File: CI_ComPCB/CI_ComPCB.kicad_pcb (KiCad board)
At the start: 2 copper layers, 145 x 101 mm, 30 parts, among them J1 Conn_01x15_Female, J10 Conn_01x02_Male, J1001 Conn_01x06_Female, J1002 Conn_01x06_Female, J1003 Conn_02x04_Odd_Even, J11 Conn_01x02_Male, J12 Conn_01x01_Female, J13 Conn_01x01_Female, J2 Conn_01x02_Male, J4 Conn_01x15_Female, J6 Conn_01x02_Male, J7 Conn_01x03_Male, J8 RJ45_LED_Shielded, J9 RJ45_LED_Shielded, Q1 IRF9540N, Q2 IRF9540N, U1 Boost_Converter, U1001 ESP32s

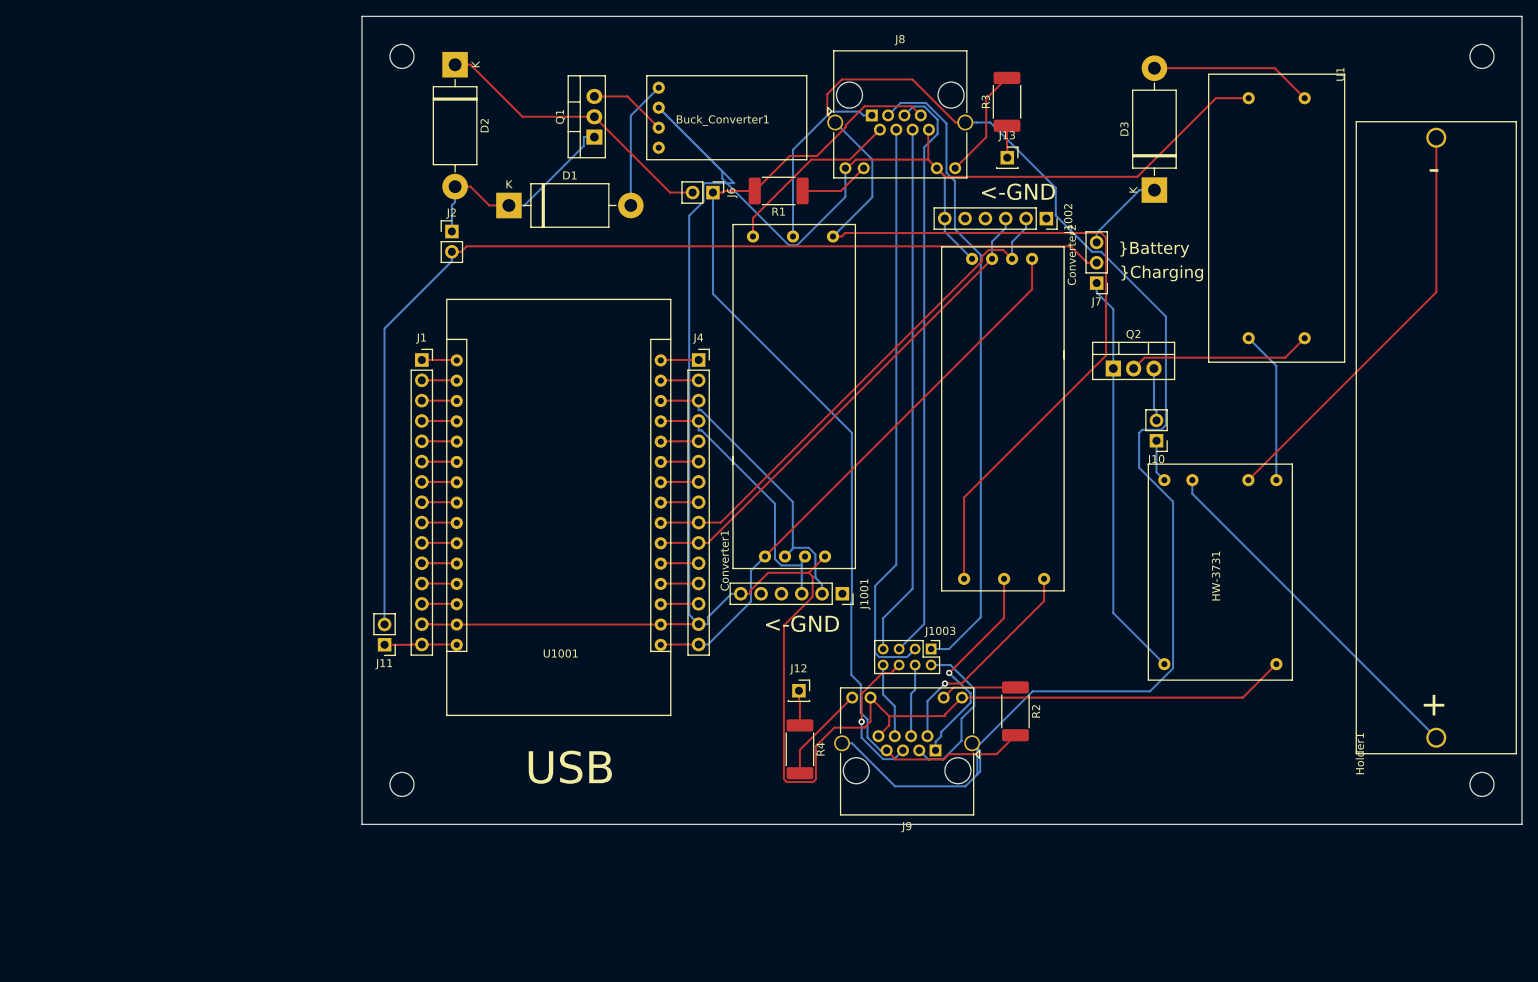
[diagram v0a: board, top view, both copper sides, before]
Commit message: Rough V1
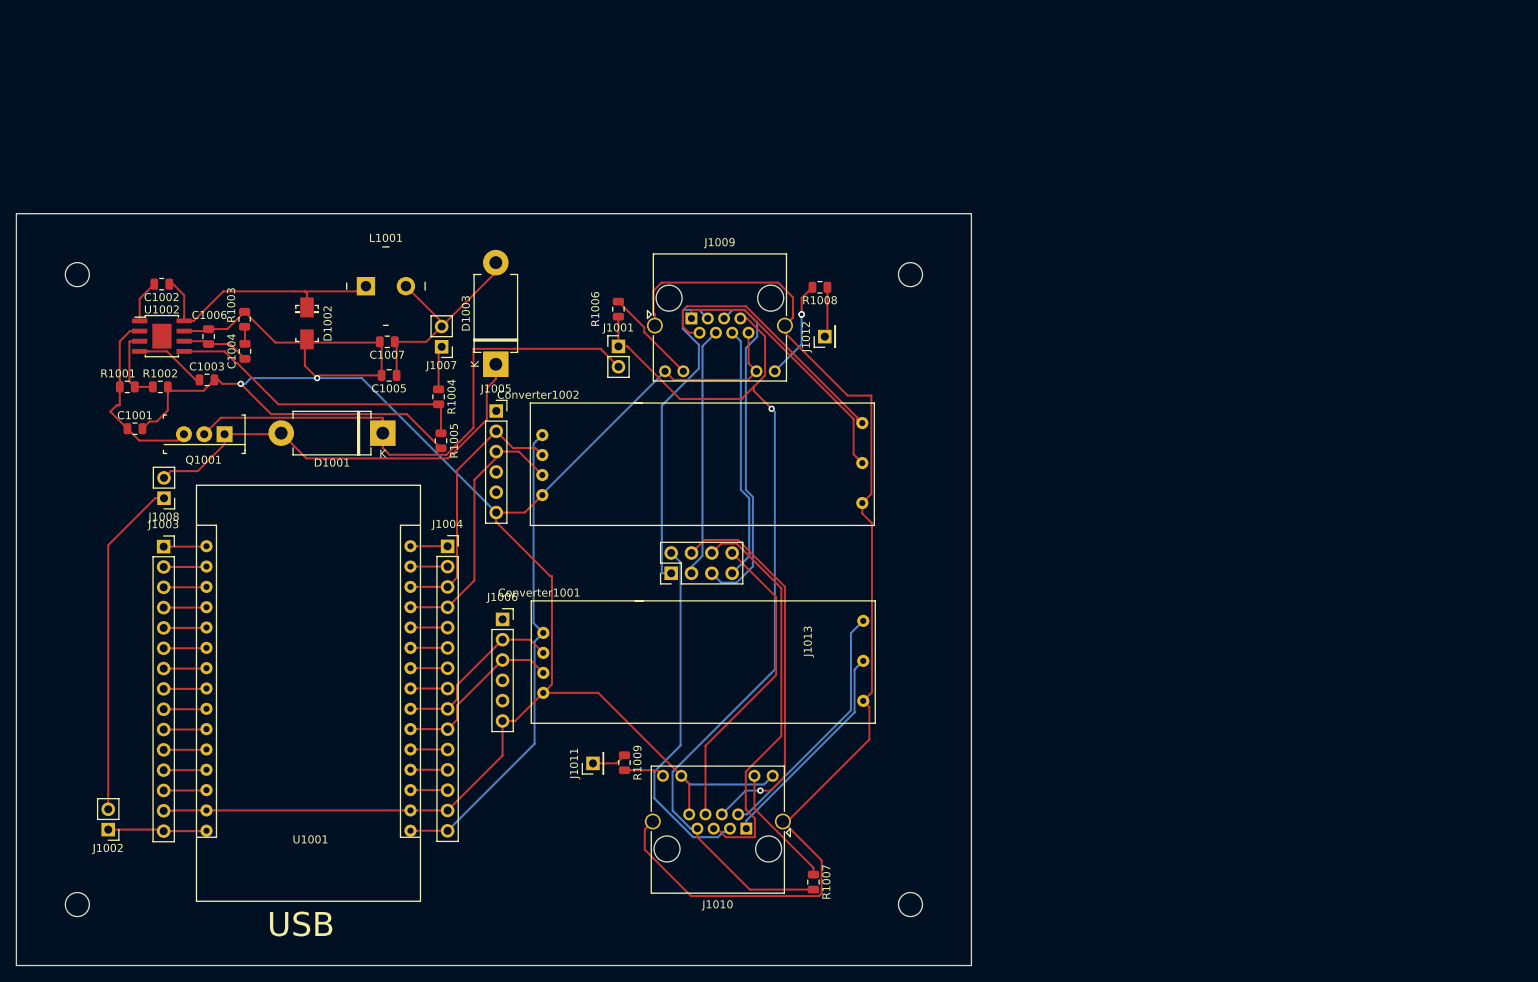
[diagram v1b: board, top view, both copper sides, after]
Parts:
- removed Buck_Converter1: 12v_to_5V, RackCom:12vto5v
- removed Converter1, Converter2: TxRx-RS485, RackCom:TXRX-AB
- removed D1, D2, D3: 1N5400, Diode_THT:D_DO-201AD_P15.24mm_Horizontal
- removed HW-3731: Charger, RackCom:Charger
- removed Holder1: Battery-New_Library, RackCom:Battery
- removed J1, J4: Conn_01x15_Female, Connector_PinSocket_2.54mm:PinSocket_1x15_P2.54mm_Vertical
- removed J10, J11, J2, J6: Conn_01x02_Male, Connector_PinHeader_2.54mm:PinHeader_1x02_P2.54mm_Vertical
- removed J12, J13: Conn_01x01_Female, Connector_PinSocket_2.54mm:PinSocket_1x01_P2.54mm_Vertical
- removed J7: Conn_01x03_Male, Connector_PinHeader_2.54mm:PinHeader_1x03_P2.54mm_Vertical
- removed J8, J9: RJ45_LED_Shielded, Connector_RJ:RJ45_Amphenol_RJHSE538X
- removed Q1, Q2: IRF9540N, Package_TO_SOT_THT:TO-220-3_Vertical
- removed R1, R2, R3, R4: 330, Resistor_SMD:R_2512_6332Metric_Pad1.52x3.35mm_HandSolder
- removed U1: Boost_Converter, RackCom:BoostConverter
- added C1001: 4700pF, Capacitor_SMD:C_0805_2012Metric, F.Cu at (65.6, 100.5)
- added C1002: 0.1uF, Capacitor_SMD:C_0805_2012Metric, F.Cu at (69.0, 82.5)
- added C1003: 0.01uF, Capacitor_SMD:C_0805_2012Metric, F.Cu at (74.6, 94.4)
- added C1004: 4700pF, Capacitor_SMD:C_0805_2012Metric, F.Cu at (79.4, 90.9)
- added C1005: 33uF, Capacitor_SMD:C_0805_2012Metric, F.Cu at (97.4, 93.9)
- added C1006: 39pF, Capacitor_SMD:C_0805_2012Metric, F.Cu at (74.8, 89.0)
- added C1007: 33uF, Capacitor_SMD:C_0805_2012Metric, F.Cu at (97.2, 89.7)
- added Converter1001: TxRx-RS485, CI_ComPCB:TXRX-AB, F.Cu at (115.2, 122.1)
- added Converter1002: TxRx-RS485, CI_ComPCB:TXRX-AB, F.Cu at (115.0, 97.3)
- added D1001: 1N5400, Diode_THT:D_DO-201AD_P12.70mm_Horizontal, F.Cu at (96.6, 101.1)
- added D1002: B340A-13-F, digikey-footprints:DO-214AC, F.Cu at (87.1, 87.4)
- added D1003: 1N5400, Diode_THT:D_DO-201AD_P12.70mm_Horizontal, F.Cu at (110.7, 92.5)
- added J1004: Conn_01x15_Female, Connector_PinSocket_2.54mm:PinSocket_1x15_P2.54mm_Vertical, F.Cu at (104.7, 115.2)
- added J1005: Conn_01x06_Female, Connector_PinSocket_2.54mm:PinSocket_1x06_P2.54mm_Vertical, F.Cu at (110.8, 98.3)
- added J1006: Conn_01x06_Female, Connector_PinSocket_2.54mm:PinSocket_1x06_P2.54mm_Vertical, F.Cu at (111.6, 124.4)
- added J1007: Conn_01x02_Male, Connector_PinHeader_2.54mm:PinHeader_1x02_P2.54mm_Vertical, F.Cu at (104.0, 90.3)
- added J1008: Conn_01x02_Male, Connector_PinHeader_2.54mm:PinHeader_1x02_P2.54mm_Vertical, F.Cu at (69.2, 109.2)
- added J1009: RJ45_LED_Shielded, Connector_RJ:RJ45_Amphenol_RJHSE538X, F.Cu at (135.2, 86.8)
- added J1010: RJ45_LED_Shielded, Connector_RJ:RJ45_Amphenol_RJHSE538X, F.Cu at (142.0, 150.5)
- added J1011: Conn_01x01_Female, Connector_PinHeader_2.54mm:PinHeader_1x01_P2.54mm_Vertical, F.Cu at (122.9, 142.4)
- added J1012: Conn_01x01_Female, Connector_PinHeader_2.54mm:PinHeader_1x01_P2.54mm_Vertical, F.Cu at (151.8, 89.0)
- added J1013: Conn_02x04_Odd_Even, Connector_PinHeader_2.54mm:PinHeader_2x04_P2.54mm_Vertical, F.Cu at (132.7, 118.6)
- added L1001: 6.8uH, digikey-footprints:Inductor_13R106C, F.Cu at (97.0, 82.7)
- added Q1001: IRF9540N, digikey-footprints:TO-220-3, F.Cu at (76.8, 101.2)
- added R1001: 332k, Resistor_SMD:R_0805_2012Metric, F.Cu at (64.7, 95.3)
- added R1002: 68.1k, Resistor_SMD:R_0805_2012Metric, F.Cu at (68.8, 95.3)
- added R1003: 44.9K, Resistor_SMD:R_0805_2012Metric, F.Cu at (79.3, 86.9)
- added R1004: 10k, Resistor_SMD:R_0805_2012Metric, F.Cu at (103.6, 96.5)
- added R1005: 1.91k, Resistor_SMD:R_0805_2012Metric, F.Cu at (103.9, 102.0)
- added R1006: 330, Resistor_SMD:R_0805_2012Metric, F.Cu at (126.0, 85.6)
- added R1007: 330, Resistor_SMD:R_0805_2012Metric, F.Cu at (150.4, 157.2)
- added R1008: 330, Resistor_SMD:R_0805_2012Metric, F.Cu at (151.2, 82.9)
- added R1009: 330, Resistor_SMD:R_0805_2012Metric, F.Cu at (126.8, 142.3)
- added U1002: TPS54331, Package_SO:TI_SO-PowerPAD-8, F.Cu at (69.0, 89.0)
- J1001, J1002: value Conn_01x06_Female -> Conn_01x02_Male; footprint Connector_PinSocket_2.54mm:PinSocket_1x06_P2.54mm_Vertical -> Connector_PinHeader_2.54mm:PinHeader_1x02_P2.54mm_Vertical
- J1003: value Conn_02x04_Odd_Even -> Conn_01x15_Female; footprint Connector_PinHeader_2.00mm:PinHeader_2x04_P2.00mm_Vertical -> Connector_PinSocket_2.54mm:PinSocket_1x15_P2.54mm_Vertical
- U1001: footprint RackCom:ESP32s -> CI_ComPCB:ESP32s
- moved J1002 139.9 mm to (62.3, 150.7), turned to 180 degrees
- moved J1003 96.8 mm to (69.2, 115.3), turned to 0 degrees
- moved J1001 41.7 mm to (126.1, 90.2), turned to 0 degrees
- moved U1001 39.0 mm to (73.3, 107.6)
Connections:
- J1001 pad 1: Net-(J1001-Pad1) -> EPower
- J1001 pad 2: TX0 -> Net-(D1001-Pad1)
- J1002 pad 2: TX2 -> Vin
- U1001 pad D12: Net-(J1-Pad12) -> Net-(J1003-Pad12)
- U1001 pad D13: Net-(J1-Pad13) -> Net-(J1003-Pad13)
- U1001 pad D14: Net-(J1-Pad11) -> Net-(J1003-Pad11)
- U1001 pad D25: Net-(J1-Pad8) -> Net-(J1003-Pad8)
- U1001 pad D26: Net-(J1-Pad9) -> Net-(J1003-Pad9)
- U1001 pad D27: Net-(J1-Pad10) -> Net-(J1003-Pad10)
- U1001 pad D32: Net-(J1-Pad6) -> Net-(J1003-Pad6)
- U1001 pad D33: Net-(J1-Pad7) -> Net-(J1003-Pad7)
- U1001 pad D34: Net-(J1-Pad4) -> Net-(J1003-Pad4)
- U1001 pad D35: Net-(J1-Pad5) -> Net-(J1003-Pad5)
- U1001 pad EN: Net-(J1-Pad1) -> Net-(J1003-Pad1)
- U1001 pad VN: Net-(J1-Pad3) -> Net-(J1003-Pad3)
- U1001 pad VP: Net-(J1-Pad2) -> Net-(J1003-Pad2)
- U1001 pad Vin: Net-(J1-Pad15) -> Net-(J1002-Pad1)
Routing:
- net Sheild: track 268.6 -> 140.5 mm
- net Vin: track 131.8 -> 42.4 mm
- net Net-(J1003-Pad1): track 80.4 -> 5.37 mm
- net Net-(D1001-Pad1): track 0.00 -> 68.9 mm
- net Net-(J1003-Pad5): track 73.4 -> 5.37 mm
- net Net-(J1003-Pad3): track 72.1 -> 5.37 mm
- net Net-(J1003-Pad7): track 66.5 -> 5.37 mm
- net Net-(D1001-Pad2): track 0.00 -> 54.1 mm
- net Net-(HW-3731-Pad2): track 52.5 -> 0.00 mm
- net Net-(HW-3731-Pad6): track 51.1 -> 0.00 mm
- net Net-(J1010-Pad5): track 0.00 -> 50.5 mm
- net Net-(J1010-Pad4): track 0.00 -> 48.6 mm, vias 0 -> 1
- net GND: track 342.6 -> 296.6 mm, vias 0 -> 2
- net Net-(HW-3731-Pad3): track 44.8 -> 0.00 mm
- net Net-(J1010-Pad3): track 0.00 -> 44.4 mm
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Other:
- board size 145 x 101 mm -> 119.4 x 94 mm
- board text removed: "+"
- board text removed: "-"
- board text removed: "<-GND"
- board text removed: "}Battery"
- board text removed: "}Charging"
